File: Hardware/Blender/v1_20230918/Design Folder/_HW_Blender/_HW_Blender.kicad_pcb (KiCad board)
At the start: 4 copper layers, 49.7 x 49.7 mm, 217 parts, among them J1001 MHDR_2POS_1.27MM_VERT, J1002 MICRO B USB_RA, J301 RCPT_4POS_1.27MM, J401 PLR237/T10BK, J402 TOTX1350(F), J501 DE-15_MALE_RA, J601 MHDR_2POS_1.27MM_VERT, J602 RCPT_4POS_1.27MM, J701 RCPT_3POS_1.27MM, J801 MHDR_2POS_1.27MM_VERT, J802 MHDR_2POS_1.27MM_VERT, J901 RCPT_6POS_2.54MM_VERT, Q1001 SI4455DY-T1-GE3, Q1002 RN1130MFV,L3F, U1001 TPS613222ADBVR, U1002 TLV74033PDBVR, U1003 MCP73811T-420I/OT, U1004 TLV74033PDBVR, U1201 MIC920YC5-TR, U1301 MIC920YC5-TR, U1401 MIC920YC5-TR, U301 STM32F446RCT6TR, U401 SN74LVC1G17DBVR, U402 SN74LVC1G17DBVR, U501 SN74LVC1G17DBVR, U502 SN74LVC1G17DBVR, U601 SN74LVC1G17DBVR, U602 ISO7720FDR, U603 SN74LVC1G17DBVR, U604 DLPT05A-7, U605 DLPT05A-7, U701 1S4E_0505S1.5U, U702 SN74LVC1G17DBVR, U703 CDSOT23-SM712, U704 MAX22028AWA+, U705 SN74LVC1G17DBVR, U801 PAM8003DR, U802 PCM1754DBQR, X301 16MHz/10ppm

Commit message: Improving the file structure and documentation
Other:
- board text removed: "RELEASED"
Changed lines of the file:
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@@
     (thickness 1.6)
   )
-  (paper "B")
+  (paper "C")
   (title_block
     (title "Blender")
@@
     (company "Mend0z0")
     (comment 1 "v1.0")
-    (comment 2 "v1.0")
+    (comment 2 "RELEASED")
     (comment 3 "Siavash Taher Parvar")
     (comment 4 "_HW_Blender.kicad_sch")
@@
     (effects (font (size 0.635 0.508) (thickness 0.127)) (justify left bottom))
   )
-  (gr_text "RELEASED" (at 145.288 88.646) (layer "Cmts.User")
-    (effects (font (size 12.7 12.7) (thickness 1.27)) (justify left bottom))
-  )
   (dimension (type aligned) (layer "Dwgs.User")

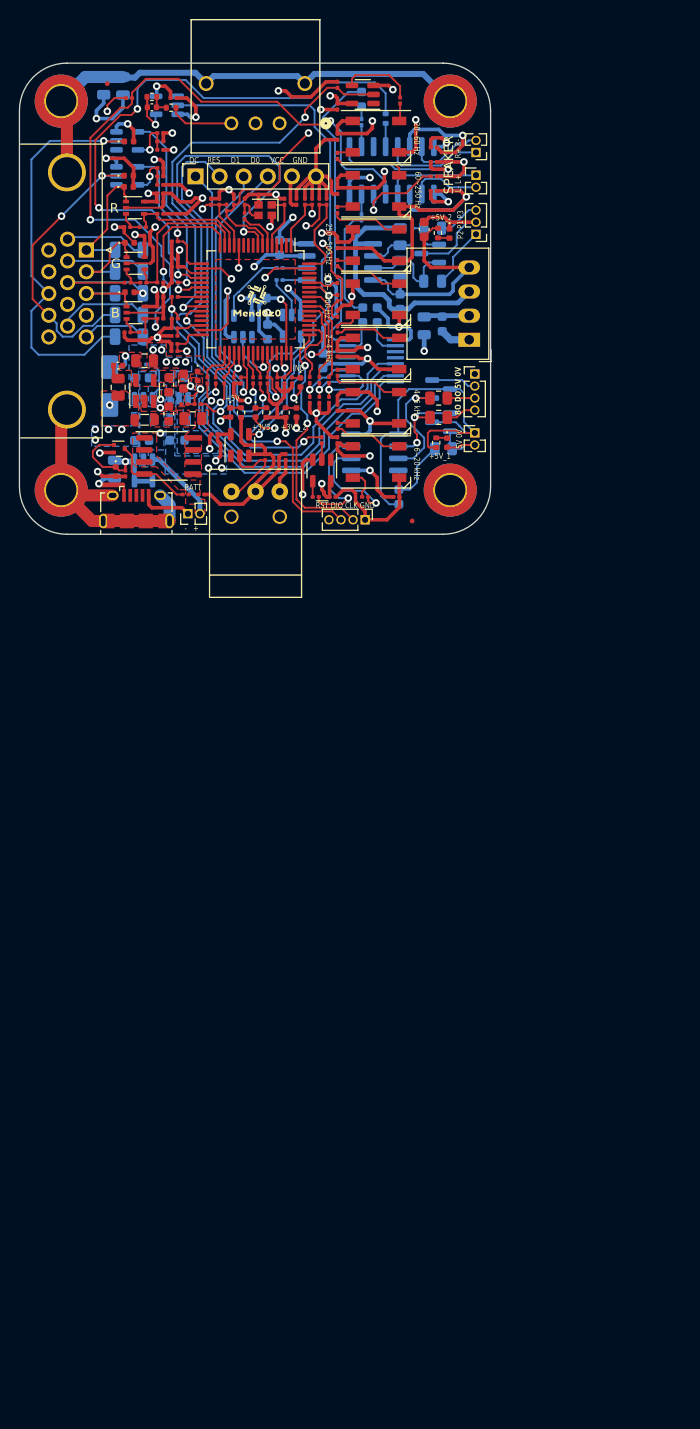
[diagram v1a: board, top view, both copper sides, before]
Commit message: More update for hardware part
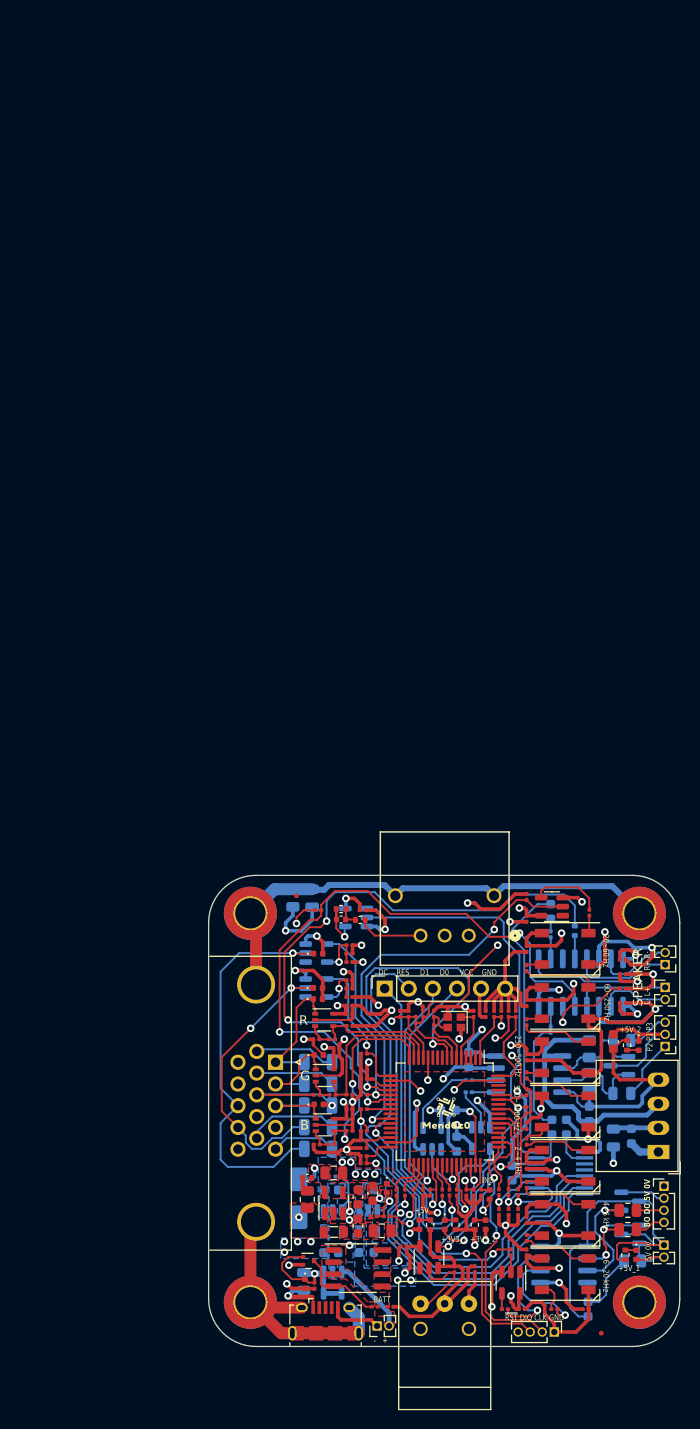
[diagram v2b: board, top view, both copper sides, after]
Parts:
- C1001, C401: value 680pF_50V -> 680pF_50V_X7R
- C1002, C1003, C1004, C1007, C1008, C1009, C1010, C610, C701, C702, C703, C704, C705, C706, C801, C802, C803, C804: value 10uF/16V -> 10uF_16V_X5R
- C1005, C1006, C301, C304, C306, C310, C312, C314, C316, C807, C901: value 1uF/6V3 -> 1uF_6V3_X5R
- C1101: value 1nF_500V -> 1nF_500V_X7R
- C1201, C1301, C1401, C308, C309, C501, C503, C601, C602, C603, C604, C605, C606, C607, C608, C609, C611, C805, C806, C808: value 2u2F/6V3 -> 2u2F_6V3_X5R
- C1202, C1302, C1402, C305, C307, C311, C313, C315, C317, C402, C403, C404, C502, C504: value 100nF/6V3 -> 100nF_6V3_X7R
- C302, C303: value 12pF/50V -> 12pF_50V_C0G
- F1001: value 0ZCK0100FF2E -> 1A_6V_0.06R
- F701, F702, F703: value 0805L010/24YR -> 0.1A_24V_1.5R
- J1001, J601, J801, J802: value MHDR_2POS_1.27MM_VERT -> MHDR_2X1_VERT_1.27MM
- J301, J602: value RCPT_4POS_1.27MM -> RECEPT_4X1_VERT_1.27MM
- J501: value DE-15_MALE_RA -> DSUB_15POS_MALE_RA
- J701: value RCPT_3POS_1.27MM -> RECEPT_3X1_VERT_1.27MM
- J901: value RCPT_6POS_2.54MM_VERT -> RECEPT_6X1_VERT_2.54MM
- L1001: value 2u2H_2A -> 2u2H_2A_0.14R
- LED1001, LED601, LED701: value GREEN -> GREEN_2V8
- LED1002, LED1003: value AMBER -> AMBER_2V
- LED301: value RED -> RED_2V
- R1001: value 4R7_1/4W -> 4R7_1/4W_1%
- R1002, R403, R812, R813, R814, R815, R901, R902: value 4K7R_1/20W -> 47KR_1/20W_1%
- R1003, R1005, R1008, R615, R701: value 470R_1/16W -> 470R_1/16W_5%
- R1004, R1007, R1203, R1303, R1403, R301, R302, R404, R504, R507, R604, R702, R801: value 10KR_1/20W -> 10KR_1/20W_1%
- R1006, R304, R601, R602, R603, R605, R606, R607, R608, R610, R613, R614, R704, R705, R803, R804, R805, R806, R807, R808, R809, R810, R811, R903, R904: value 100R_1/20W -> 100R_1/20W_1%
- R1101: value 1MR_1/2W -> 1MR_1/2W_5%
- R1201, R1202, R1301, R1302, R1401, R1402: value 47KR_1/20W -> 4K7R_1/20W_1%
- R303, R506, R509: value 49R9_1/20W -> 49R9_1/20W_1%
- R401: value 330R_1/16W -> 330R_1/16W_1%
- R402, R802: value 100R_1/10W -> 100R_1/10W_1%
- R501, R502, R503, R505, R508: value 75R_2W -> 75R_2W_1%
- R609: value 100R_1/8W -> 100R_1/8W_5%
- R611, R612: value 1KR_1/8W -> 1KR_1/8W_5%
- R703, R706: value 680R_1/8W -> 680R_1/8W_5%
- RV1001, RV1002: value PTC_500mA -> 0.5A_6V_0.15R
- X301: value 16MHz/10ppm -> 16MHz_12pF_10ppm
- moved C301 87.9 mm to (143.1, 211.2)
- moved C302 87.9 mm to (148.5, 211.2)
- moved C303 87.9 mm to (144.3, 211.2)
- moved C304 87.9 mm to (151.4, 211.2)
- moved C305 87.9 mm to (150.6, 211.2)
- moved C306 87.9 mm to (140.7, 211.2)
- moved C307 87.9 mm to (141.6, 211.2)
- moved C316 87.9 mm to (152.1, 211.2)
- moved C317 87.9 mm to (152.9, 211.2)
- moved C404 87.9 mm to (136.8, 200.3)
- moved C602 87.9 mm to (154.1, 210.1)
- moved C808 87.9 mm to (164.2, 210.1)
- moved C901 87.9 mm to (149.7, 211.2)
- moved D602 87.9 mm to (158.1, 210.1)
- moved FD1101 87.9 mm to (129.8, 198.8)
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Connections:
- net /BLOCK DIAGRAM/ISOLATED VGA INPUT/DB_HSYNC renamed /BLOCK DIAGRAM/BUFFERED VGA INPUT/DB_HSYNC
- net /BLOCK DIAGRAM/ISOLATED VGA INPUT/DB_SIG_BLUE renamed /BLOCK DIAGRAM/BUFFERED VGA INPUT/DB_SIG_BLUE
- net /BLOCK DIAGRAM/ISOLATED VGA INPUT/DB_SIG_GREEN renamed /BLOCK DIAGRAM/BUFFERED VGA INPUT/DB_SIG_GREEN
- net /BLOCK DIAGRAM/ISOLATED VGA INPUT/DB_SIG_RED renamed /BLOCK DIAGRAM/BUFFERED VGA INPUT/DB_SIG_RED
- net /BLOCK DIAGRAM/ISOLATED VGA INPUT/DB_VSYNC renamed /BLOCK DIAGRAM/BUFFERED VGA INPUT/DB_VSYNC
- net /BLOCK DIAGRAM/ISOLATED VGA INPUT/VID_SIG_B renamed /BLOCK DIAGRAM/BUFFERED VGA INPUT/VID_SIG_B
- net /BLOCK DIAGRAM/ISOLATED VGA INPUT/VID_SIG_G renamed /BLOCK DIAGRAM/BUFFERED VGA INPUT/VID_SIG_G
- net /BLOCK DIAGRAM/ISOLATED VGA INPUT/VID_SIG_HSYNC renamed /BLOCK DIAGRAM/BUFFERED VGA INPUT/VID_SIG_HSYNC
- net /BLOCK DIAGRAM/ISOLATED VGA INPUT/VID_SIG_R renamed /BLOCK DIAGRAM/BUFFERED VGA INPUT/VID_SIG_R
- net /BLOCK DIAGRAM/ISOLATED VGA INPUT/VID_SIG_VSYNC renamed /BLOCK DIAGRAM/BUFFERED VGA INPUT/VID_SIG_VSYNC
- net /BLOCK DIAGRAM/MCU/+3V3_1 renamed /BLOCK DIAGRAM/MICROCONTROLLER/+3V3_1
- net /BLOCK DIAGRAM/MCU/EN_PWR renamed /BLOCK DIAGRAM/MICROCONTROLLER/EN_PWR
- net /BLOCK DIAGRAM/MCU/I2S_CK renamed /BLOCK DIAGRAM/MICROCONTROLLER/I2S_CK
- net /BLOCK DIAGRAM/MCU/I2S_MCK renamed /BLOCK DIAGRAM/MICROCONTROLLER/I2S_MCK
- net /BLOCK DIAGRAM/MCU/I2S_SD renamed /BLOCK DIAGRAM/MICROCONTROLLER/I2S_SD
- net /BLOCK DIAGRAM/MCU/I2S_WS renamed /BLOCK DIAGRAM/MICROCONTROLLER/I2S_WS
- net /BLOCK DIAGRAM/MCU/MCU_BOOT0 renamed /BLOCK DIAGRAM/MICROCONTROLLER/MCU_BOOT0
- net /BLOCK DIAGRAM/MCU/MCU_LED renamed /BLOCK DIAGRAM/MICROCONTROLLER/MCU_LED
- net /BLOCK DIAGRAM/MCU/MCU_OSC_I renamed /BLOCK DIAGRAM/MICROCONTROLLER/MCU_OSC_I
- net /BLOCK DIAGRAM/MCU/MCU_OSC_O renamed /BLOCK DIAGRAM/MICROCONTROLLER/MCU_OSC_O
- net /BLOCK DIAGRAM/MCU/MCU_SWCLK renamed /BLOCK DIAGRAM/MICROCONTROLLER/MCU_SWCLK
- net /BLOCK DIAGRAM/MCU/MCU_SWDIO renamed /BLOCK DIAGRAM/MICROCONTROLLER/MCU_SWDIO
- net /BLOCK DIAGRAM/MCU/MCU_VCAP renamed /BLOCK DIAGRAM/MICROCONTROLLER/MCU_VCAP
- net /BLOCK DIAGRAM/MCU/MCU_~{NRST} renamed /BLOCK DIAGRAM/MICROCONTROLLER/MCU_~{NRST}
- net /BLOCK DIAGRAM/MCU/PAM8003_~{SHDN} renamed /BLOCK DIAGRAM/SPEAKER DRIVER/PAM8003_~{SHDN}
- net /BLOCK DIAGRAM/MCU/PCM1754_DEMP renamed /BLOCK DIAGRAM/MICROCONTROLLER/PCM1754_DEMP
- net /BLOCK DIAGRAM/MCU/PCM1754_FMT renamed /BLOCK DIAGRAM/MICROCONTROLLER/PCM1754_FMT
- net /BLOCK DIAGRAM/MCU/PCM1754_MUTE renamed /BLOCK DIAGRAM/MICROCONTROLLER/PCM1754_MUTE
- net /BLOCK DIAGRAM/MCU/TOSLINK_DATA renamed /BLOCK DIAGRAM/MICROCONTROLLER/TOSLINK_DATA
- net /BLOCK DIAGRAM/SPEAKER DRIVER/SPKL+ renamed /BLOCK DIAGRAM/SPEAKER DRIVER/PAM8003_SPKL+
- net /BLOCK DIAGRAM/SPEAKER DRIVER/SPKL- renamed /BLOCK DIAGRAM/SPEAKER DRIVER/PAM8003_SPKL-
- net /BLOCK DIAGRAM/SPEAKER DRIVER/SPKR+ renamed /BLOCK DIAGRAM/SPEAKER DRIVER/PAM8003_SPKR+
- net /BLOCK DIAGRAM/SPEAKER DRIVER/SPKR- renamed /BLOCK DIAGRAM/SPEAKER DRIVER/PAM8003_SPKR-
- net Net-(U801-INL) renamed /BLOCK DIAGRAM/SPEAKER DRIVER/PAM8003_INL
- net Net-(U801-INR) renamed /BLOCK DIAGRAM/SPEAKER DRIVER/PAM8003_INR
- net Net-(U802-BCK) renamed /BLOCK DIAGRAM/SPEAKER DRIVER/PCM_BCK
- net Net-(U802-DATA) renamed /BLOCK DIAGRAM/SPEAKER DRIVER/PCM_DATA
- net Net-(U802-DEMP) renamed /BLOCK DIAGRAM/SPEAKER DRIVER/PCM_DEMP
- net Net-(U802-FMT) renamed /BLOCK DIAGRAM/SPEAKER DRIVER/PCM_FMT
- net Net-(U802-LRCK) renamed /BLOCK DIAGRAM/SPEAKER DRIVER/PCM_LRCK
- net Net-(U802-MUTE) renamed /BLOCK DIAGRAM/SPEAKER DRIVER/PCM_MUTE
- net Net-(U802-SCK) renamed /BLOCK DIAGRAM/SPEAKER DRIVER/PCM_SCK
- net Net-(U802-V_L_OUT) renamed /BLOCK DIAGRAM/SPEAKER DRIVER/PCM_L_OUT
- net Net-(U802-V_R_OUT) renamed /BLOCK DIAGRAM/SPEAKER DRIVER/PCM_R_OUT
- R802 pad 1: /BLOCK DIAGRAM/MCU/PAM8003_VOLUME -> /BLOCK DIAGRAM/SPEAKER DRIVER/PAM8003_VOLUME
- R802 pad 2: Net-(U801-VOLUME) -> /BLOCK DIAGRAM/SPEAKER DRIVER/PAM8003_VOLUME
- U301 pad 20: /BLOCK DIAGRAM/MCU/PAM8003_VOLUME -> /BLOCK DIAGRAM/SPEAKER DRIVER/PAM8003_VOLUME
- U801 pad 12: Net-(U801-VOLUME) -> /BLOCK DIAGRAM/SPEAKER DRIVER/PAM8003_VOLUME
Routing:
- net /BLOCK DIAGRAM/SPEAKER DRIVER/PAM8003_VOLUME: track 0.00 -> 64.6 mm, vias 0 -> 3
- net /BLOCK DIAGRAM/MCU/PAM8003_VOLUME: track 62.2 -> 0.00 mm, vias 3 -> 0
- net Net-(U801-VOLUME): track 2.45 -> 0.00 mm
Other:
- board text added: "correct the dating format!"

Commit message: Updating README.md
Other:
- board text removed: "correct the dating format!"
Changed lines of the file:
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@@
     (effects (font (size 0.635 0.508) (thickness 0.127)) (justify left bottom))
-  )
-  (gr_text "correct the dating format!" (at 176.149 237.3695) (layer "Cmts.User")
-    (effects (font (size 2.54 2.54) (thickness 0.15)) (justify left bottom))
   )
   (dimension (type aligned) (layer "Dwgs.User")
